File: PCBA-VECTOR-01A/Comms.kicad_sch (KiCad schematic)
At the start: 33 parts, among them J1 Screw_Terminal_01x06, J16 Conn_01x02_Pin, J18 Screw_Terminal_01x03, J20 Conn_01x02_Pin, J21 Screw_Terminal_01x03, J6 Conn_01x03_Pin, J8 Screw_Terminal_01x04, U10 NUP4114, U11 NUP4114, U12 MCP2551-I-SN, U14 ST485EDR, U17 TYPE-C 16PLT-H10.0, U9 NUP4114

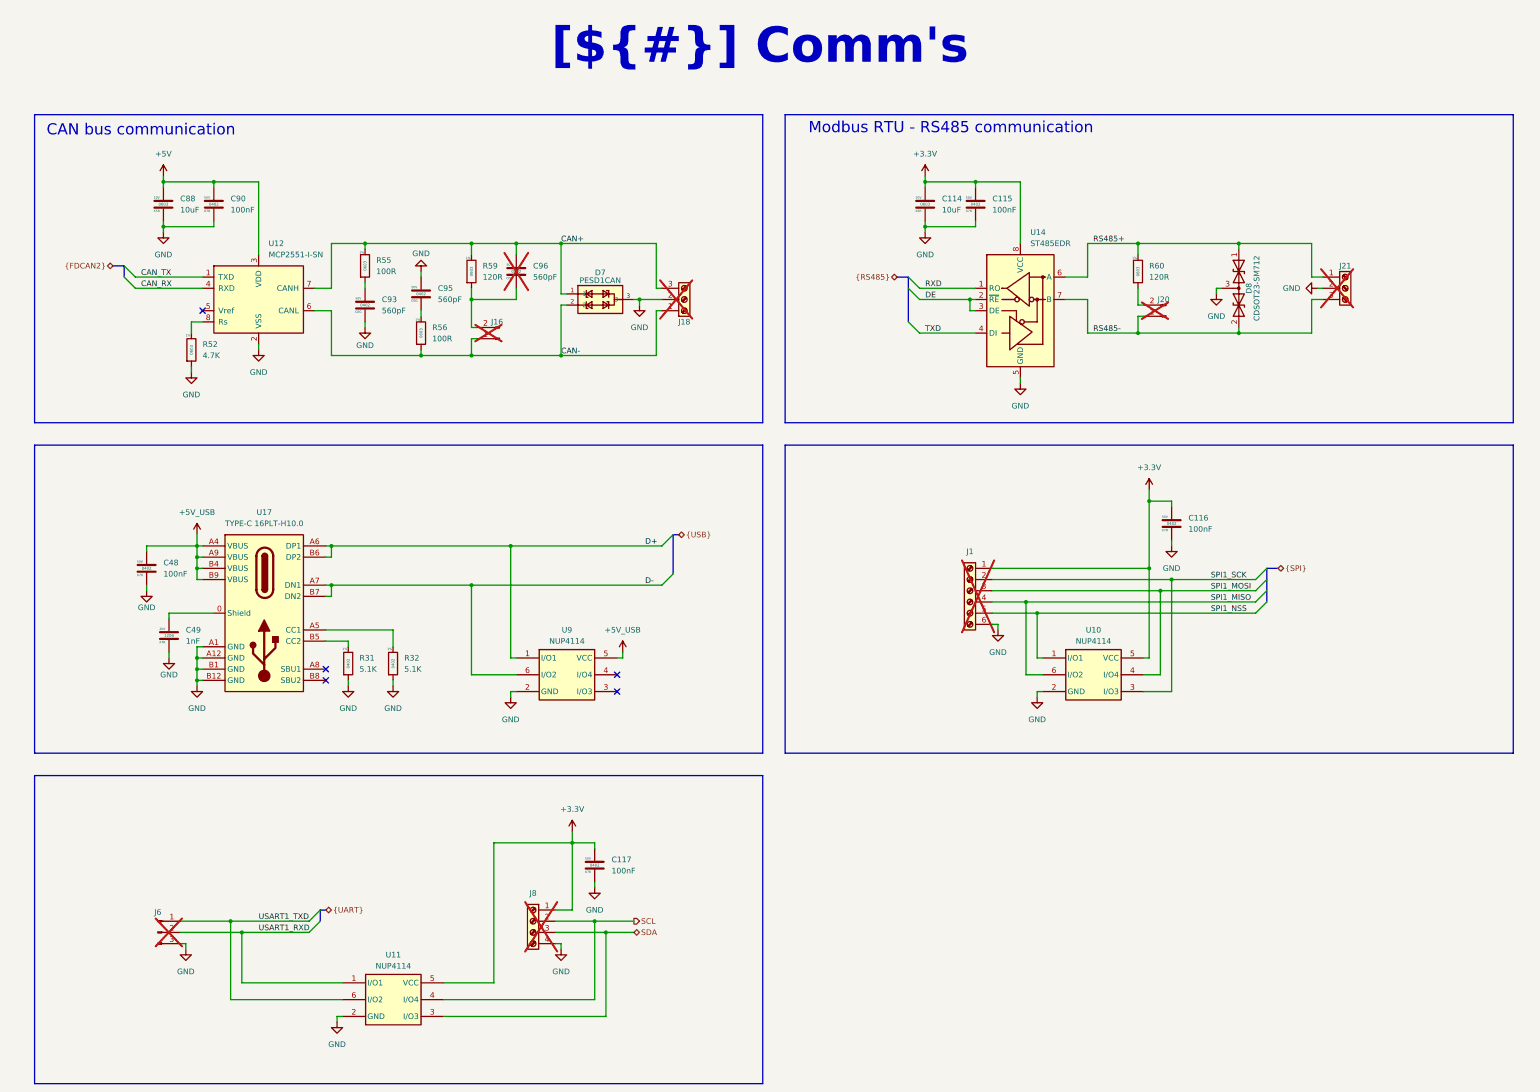
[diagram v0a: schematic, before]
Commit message: Finished schematic?
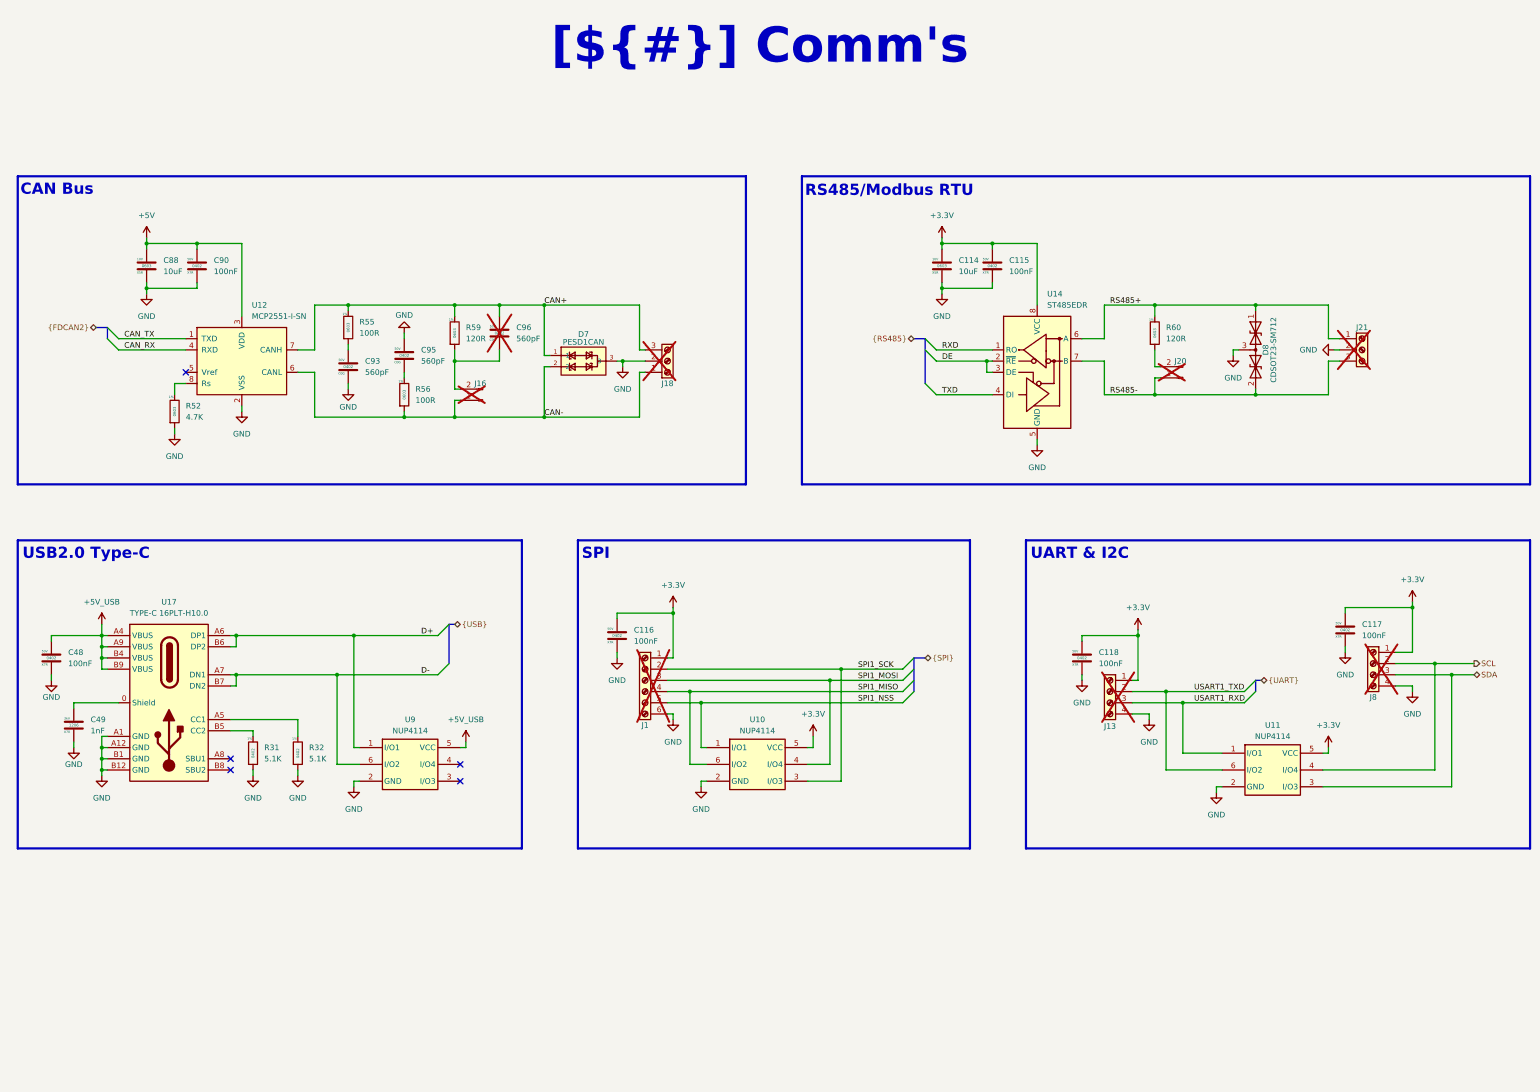
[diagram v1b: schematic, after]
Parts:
- removed J6: Conn_01x03_Pin, Connector_PinHeader_2.54mm:PinHeader_1x03_P2.54mm_Vertical, symbol Connector:Conn_01x03_Pin
- added C118: 100nF, Capacitor_SMD:C_0402_1005Metric, symbol Device:C
- added J13: Screw_Terminal_01x04, Bvrny's_library:TerminalBlock_5.08_01x04_JLAB, symbol Connector:Screw_Terminal_01x04
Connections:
- net +3.3V: now also C118.1, J13.1 (Pin_1)
- net GND: now also C118.2, J13.4 (Pin_4)
- net USART1_RXD: now also J13.3 (Pin_3)
- net USART1_TXD: now also J13.2 (Pin_2)
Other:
- note added: "CAN Bus"
- note added: "RS485/Modbus RTU"
- note added: "SPI"
- note added: "UART & I2C"
- note added: "USB2.0 Type-C"
- note removed: "CAN bus communication"
- note removed: "Modbus RTU - RS485 communication"
- moved on the sheet: C114, C115, C116, C117, C48, C49, C88, C90, C93, C95, C96, D7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
